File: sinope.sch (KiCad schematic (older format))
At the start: 36 parts, among them J1 5VDC, J2 PIOA, J3 PIOB, J4 SERIAL0, J5 SERIAL1, J6 Battery, Q1 2N3904, U1 74LS04, U10 Z80PIO, U11 Z80SIO, U12 MAX232, U13 MAX232, U2 Z80CPU, U3 74LS32, U5 27128, U6 74LS138, U7 MAX695, U8 Z80CTC, U9 TC551001, Y1 3.6864

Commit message: Video interface
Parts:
- added C14, C17, C18, C19, C20, C21: 100nF, symbol Device:C_Small
- added C15, C16: 16pF, symbol Device:C_Small
- added U14: TMS9929A, symbol sinope:TMS9929A
- added U15, U16, U18: 74HCT574, symbol 74xx:74HCT574
- added U17: HM62256BLP-7, DIP28, symbol sinope:HM62256BLP-7
- added U19: 74HCT04, symbol 74xx:74HCT04
- added U4: 74LS32, Package_DIP:DIP-14_W7.62mm, symbol 74xx:74LS32
- added Y2: 10.738635MHz, Crystal:Crystal_HC49-U_Horizontal, symbol Device:Crystal
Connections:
- net labels added: AD0, AD1, AD2, AD3, AD4, AD5, AD6, AD7, RD0, RD1, RD2, RD3, RD4, RD5, RD6, RD7, VA0, VA1, VA10, VA11, VA12, VA13, VA14, VA2, VA3, VA4, VA5, VA6, VA7, VA8, VA9, VIDEO_ADDRESS, VIDEO_DATA, ~NMI, ~VIDEOCS, ~WR
- wire segments 355 -> 548
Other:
- moved on the sheet: C10, C11, C12, C13, C4, C5, C6, C7, C8, C9, J4, J5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

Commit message: Rip out graphics
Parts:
- removed C16: 16pF, symbol Device:C_Small
- removed C17, C18, C19, C20, C21: 100nF, symbol Device:C_Small
- removed unit 2 of U1
- removed U14: TMS9929A, symbol sinope:TMS9929A
- removed U15, U16, U18: 74HCT574, symbol 74xx:74HCT574
- removed U17: HM62256BLP-7, DIP28, symbol sinope:HM62256BLP-7
- removed U19: 74HCT04, symbol 74xx:74HCT04
- removed U3, U4: 74LS32, Package_DIP:DIP-14_W7.62mm, symbol 74xx:74LS32
- removed U6: 74LS138, Package_DIP:DIP-16_W7.62mm, symbol 74xx:74LS138
- removed Y2: 10.738635MHz, Crystal:Crystal_HC49-U_Horizontal, symbol Device:Crystal
- added U3: SINOPE_GAL, symbol sinope:SINOPE_GAL
- C15: value 16pF -> 100nF
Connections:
- net labels added: CTSA, RAMVCC, RTSA, RxDA, TxDA, ~CTCCS, ~INT, ~MREQ, ~PIOCS, ~RAMCS, ~RAMCS_SAFE, ~ROMCS, ~SIOCS
- net labels removed: AD0, AD1, AD2, AD3, AD4, AD5, AD6, AD7, ADDRESS, DATA, RD0, RD1, RD2, RD3, RD4, RD5, RD6, RD7, VA0, VA1, VA10, VA11, VA12, VA13, VA14, VA2, VA3, VA4, VA5, VA6, VA7, VA8, VA9, VIDEO_ADDRESS, VIDEO_DATA, ~NMI, ~VIDEOCS
- wire segments 548 -> 345
- no-connect marks 41 -> 36
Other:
- moved on the sheet: C1, C10, C11, C12, C13, C4, C5, C6, C7, C8, C9, J1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

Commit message: Use integrated oscillator
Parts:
- removed C2, C3: 47pF, Capacitor_SMD:C_0805_2012Metric, symbol Device:C
- removed R3: 10M, Resistor_SMD:R_0805_2012Metric, symbol Device:R
- removed R4: 1k, Resistor_SMD:R_0805_2012Metric, symbol Device:R
- removed U1: 74LS04, Package_DIP:DIP-14_W7.62mm, symbol 74xx:74LS04
- removed Y1: 3.6864, Crystal:Crystal_HC49-U_Horizontal, symbol Device:Crystal
- added X1: 3.6864Mhz, Oscillator:Oscillator_DIP-14, symbol Oscillator:TFT680
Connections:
- wire segments 345 -> 337
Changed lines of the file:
@@
 Text GLabel 2900 7150 2    50   Output ~ 0
 ~RESET
-$Comp
-L Device:C C2
-U 1 1 5EAE2B1A
-P 2250 1500
-F 0 "C2" H 2365 1546 50  0000 L CNN
-F 1 "47pF" H 2365 1455 50  0000 L CNN
-F 2 "Capacitor_SMD:C_0805_2012Metric" H 2288 1350 50  0001 C CNN
-F 3 "~" H 2250 1500 50  0001 C CNN
-	1    2250 1500
-	1    0    0    -1
-$EndComp
-$Comp
-L Device:C C3
-U 1 1 5EAE32B1
-P 2800 1500
-F 0 "C3" H 2915 1546 50  0000 L CNN
-F 1 "47pF" H 2915 1455 50  0000 L CNN
-F 2 "Capacitor_SMD:C_0805_2012Metric" H 2838 1350 50  0001 C CNN
-F 3 "~" H 2800 1500 50  0001 C CNN
-	1    2800 1500
-	1    0    0    -1
-$EndComp
-$Comp
-L Device:R R3
-U 1 1 5EAE40DE
-P 2250 1000
-F 0 "R3" H 2050 1050 50  0000 L CNN
-F 1 "10M" H 2050 950 50  0000 L CNN
-F 2 "Resistor_SMD:R_0805_2012Metric" V 2180 1000 50  0001 C CNN
-F 3 "~" H 2250 1000 50  0001 C CNN
-	1    2250 1000
-	1    0    0    -1
-$EndComp
-$Comp
-L Device:R R4
-U 1 1 5EAE4756
-P 2800 1000
-F 0 "R4" H 2870 1046 50  0000 L CNN
-F 1 "1k" H 2870 955 50  0000 L CNN
-F 2 "Resistor_SMD:R_0805_2012Metric" V 2730 1000 50  0001 C CNN
-F 3 "~" H 2800 1000 50  0001 C CNN
-	1    2800 1000
-	1    0    0    -1
-$EndComp
-$Comp
-L Device:Crystal Y1
-U 1 1 5EAE53AE
-P 2550 1250
-F 0 "Y1" H 2550 1518 50  0000 C CNN
-F 1 "3.6864" H 2550 1427 50  0000 C CNN
-F 2 "Crystal:Crystal_HC49-U_Horizontal" H 2550 1250 50  0001 C CNN
-F 3 "~" H 2550 1250 50  0001 C CNN
-	1    2550 1250
-	1    0    0    -1
-$EndComp
-$Comp
-L 74xx:74LS04 U1
-U 1 1 5EAED368
-P 1850 1250
-F 0 "U1" H 1850 1550 50  0000 C CNN
-F 1 "74LS04" H 1850 1450 50  0000 C CNN
-F 2 "Package_DIP:DIP-14_W7.62mm" H 1850 1250 50  0001 C CNN
-F 3 "http://www.ti.com/lit/gpn/sn74LS04" H 1850 1250 50  0001 C CNN
-	1    1850 1250
-	-1   0    0    1
-$EndComp
-Wire Wire Line
-	1550 1250 1550 2600
 Wire Wire Line
 	1550 2600 1850 2600
-Wire Wire Line
-	2150 1250 2250 1250
-Wire Wire Line
-	2250 1250 2250 1150
-Connection ~ 2250 1250
-Wire Wire Line
-	2250 1250 2400 1250
-Wire Wire Line
-	2250 1350 2250 1250
-Wire Wire Line
-	2700 1250 2800 1250
-Wire Wire Line
-	2800 1250 2800 1150
-Wire Wire Line
-	2800 1250 2800 1350
-Connection ~ 2800 1250
-Wire Wire Line
-	2250 1650 2800 1650
-$Comp
-L power:GND #PWR09
-U 1 1 5EB1616A
-P 2800 1650
-F 0 "#PWR09" H 2800 1400 50  0001 C CNN
-F 1 "GND" H 2805 1477 50  0000 C CNN
-F 2 "" H 2800 1650 50  0001 C CNN
-F 3 "" H 2800 1650 50  0001 C CNN
-	1    2800 1650
-	1    0    0    -1
-$EndComp
-Wire Wire Line
-	1550 1250 1550 750
-Wire Wire Line
-	1550 750  2250 750
-Wire Wire Line
-	2250 750  2250 850
-Connection ~ 1550 1250
-Wire Wire Line
-	2250 750  2800 750
-Wire Wire Line
-	2800 750  2800 850
-Connection ~ 2250 750
-Connection ~ 2800 1650
 Text GLabel 1800 3300 0    50   Output ~ 0
 ~M1
-Text GLabel 1000 1250 0    50   Output ~ 0
+Text GLabel 1650 1250 2    50   Output ~ 0
 CLK
-Wire Wire Line
-	1000 1250 1550 1250
 Entry Wire Line
 	3750 2200 3650 2300
@@
 Wire Wire Line
 	4900 4200 4900 4250
+$Comp
+L power:GND #PWR03
+U 1 1 5F85FCD9
+P 1250 1600
+F 0 "#PWR03" H 1250 1350 50  0001 C CNN
+F 1 "GND" H 1255 1427 50  0000 C CNN
+F 2 "" H 1250 1600 50  0001 C CNN
+F 3 "" H 1250 1600 50  0001 C CNN
+	1    1250 1600
+	1    0    0    -1
+$EndComp
+$Comp
+L power:+5V #PWR02
+U 1 1 5F860570
+P 1250 900
+F 0 "#PWR02" H 1250 750 50  0001 C CNN
+F 1 "+5V" H 1265 1073 50  0000 C CNN
+F 2 "" H 1250 900 50  0001 C CNN
+F 3 "" H 1250 900 50  0001 C CNN
+	1    1250 900
+	1    0    0    -1
+$EndComp
+$Comp
+L Oscillator:TFT680 X1
+U 1 1 5F81E577
+P 1250 1250
+F 0 "X1" H 1550 1600 50  0000 L CNN
+F 1 "3.6864Mhz" H 1400 1500 50  0000 L CNN
+F 2 "Oscillator:Oscillator_DIP-14" H 1700 900 50  0001 C CNN
+F 3 "http://cdn-reichelt.de/documents/datenblatt/B400/OSZI.pdf" H 1150 1250 50  0001 C CNN
+	1    1250 1250
+	1    0    0    -1
+$EndComp
+Wire Wire Line
+	1250 900  1250 950
+Wire Wire Line
+	1250 900  900  900
+Wire Wire Line
+	900  900  900  1250
+Wire Wire Line
+	900  1250 950  1250
+Connection ~ 1250 900
+Wire Wire Line
+	1550 1250 1550 2600
+Wire Wire Line
+	1550 1250 1650 1250
+Connection ~ 1550 1250
+Wire Wire Line
+	1250 1600 1250 1550
 Wire Bus Line
 	3650 2300 3650 3950

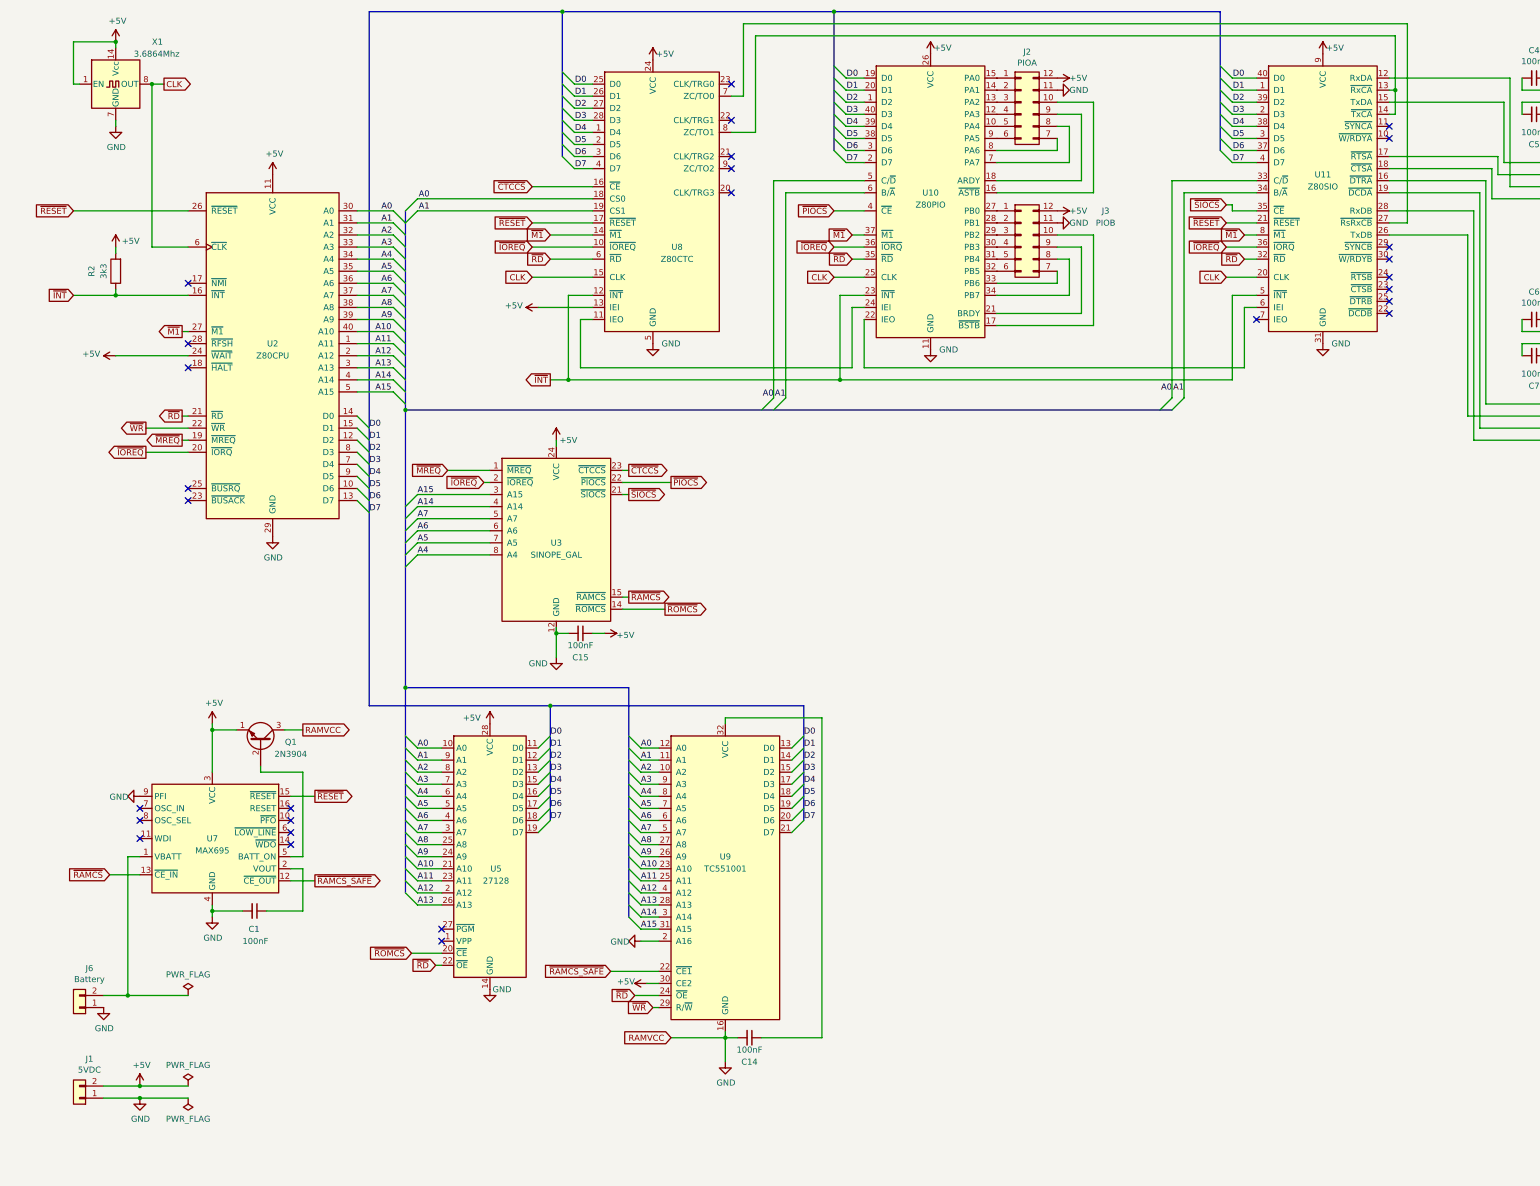
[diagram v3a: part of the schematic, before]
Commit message: Touchup
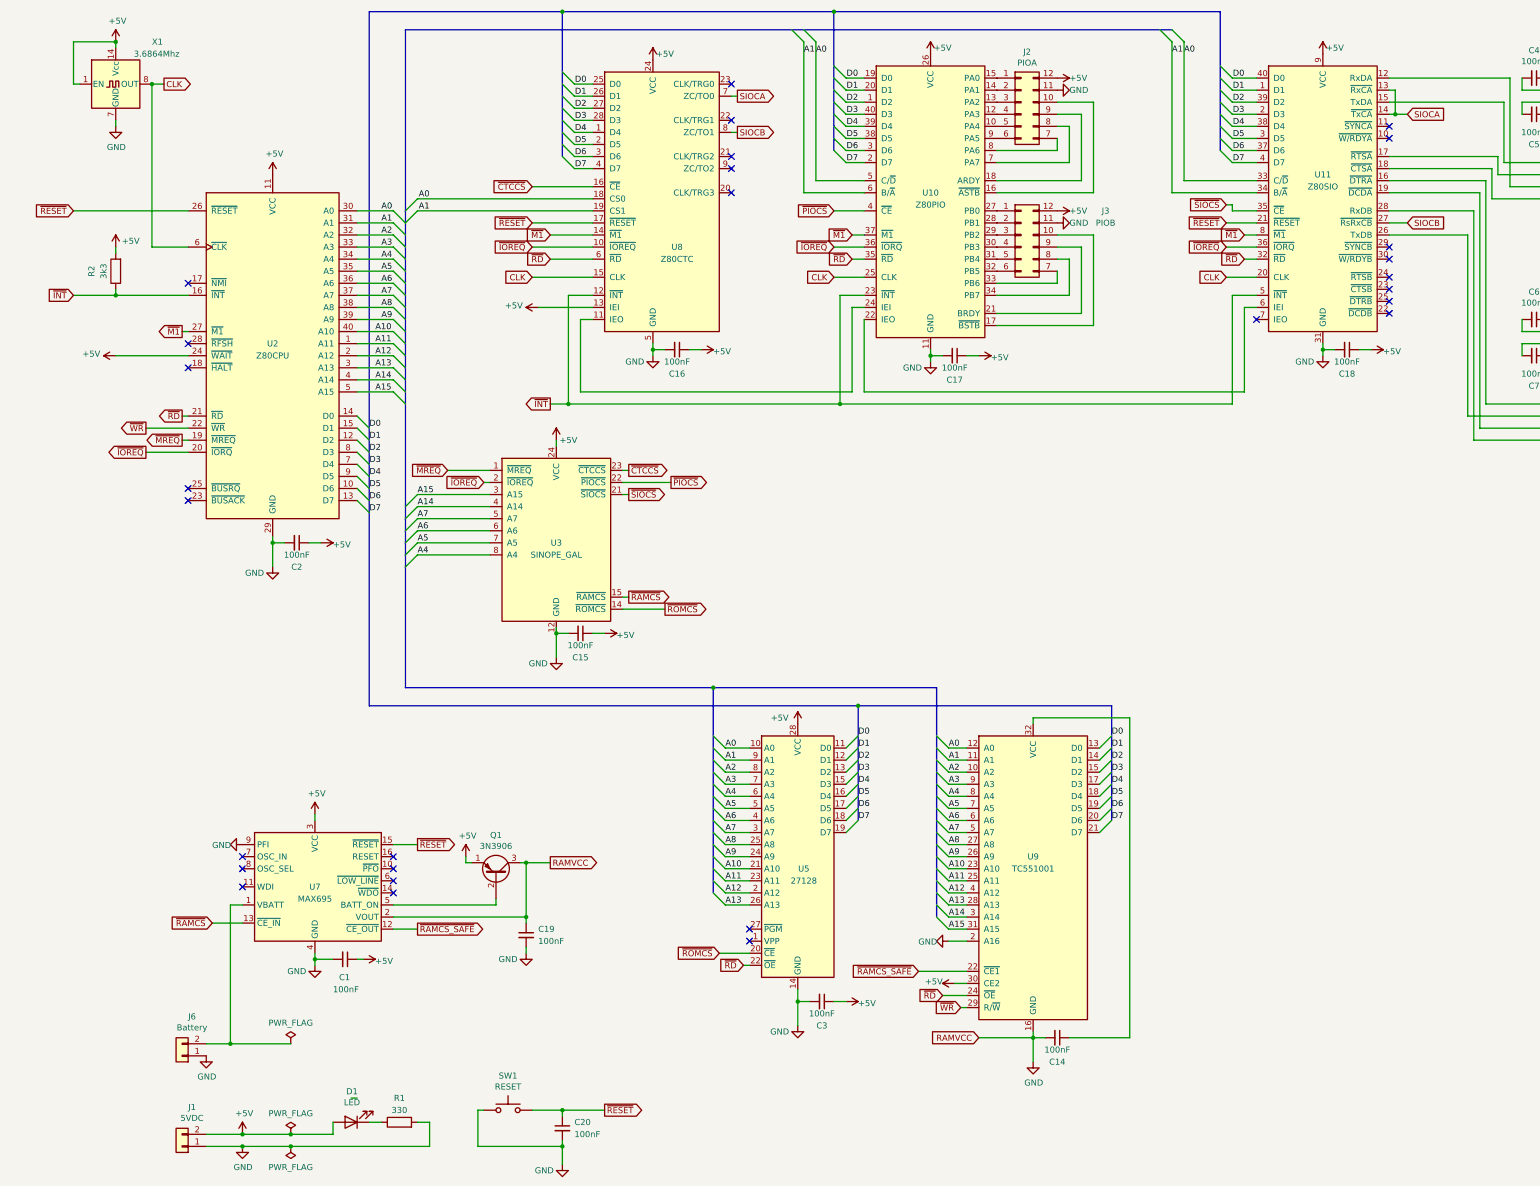
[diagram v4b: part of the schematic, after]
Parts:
- removed Q1: 2N3904, Package_TO_SOT_THT:TO-92_Inline, symbol Transistor_BJT:2N3904
- added C16, C17, C18, C19, C2, C20, C3: 100nF, Capacitor_SMD:C_0805_2012Metric, symbol Device:C_Small
- added D1: LED, LED_SMD:LED_0805_2012Metric, symbol Device:LED
- added Q1: 3N3906, Package_TO_SOT_THT:TO-92, symbol Device:Q_PNP_EBC
- added R1: 330, Resistor_SMD:R_0805_2012Metric, symbol Device:R
- added SW1: RESET, Button_Switch_THT:Push_E-Switch_KS01Q01, symbol Switch:SW_Push
- C1, C14, C15: footprint (none) -> Capacitor_SMD:C_0805_2012Metric
- J1: footprint (none) -> Connector_PinHeader_2.54mm:PinHeader_1x02_P2.54mm_Vertical
- J6: footprint (none) -> Connector_PinHeader_2.54mm:PinHeader_2x01_P2.54mm_Vertical
- R2: footprint (none) -> Resistor_SMD:R_0805_2012Metric
- U3: footprint (none) -> Package_DIP:DIP-24_W7.62mm
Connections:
- net labels added: SIOCA, SIOCB
- wire segments 337 -> 368
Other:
- moved on the sheet: C1, C14, J1, J6, U5, U7, U9
